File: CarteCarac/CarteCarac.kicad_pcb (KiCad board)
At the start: 4 copper layers, 250 x 130 mm, 30 parts, among them J1 Conn_02x25_Top_Bottom_Mountin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, J2 Conn_02x39_Top_Bottom_Mountin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

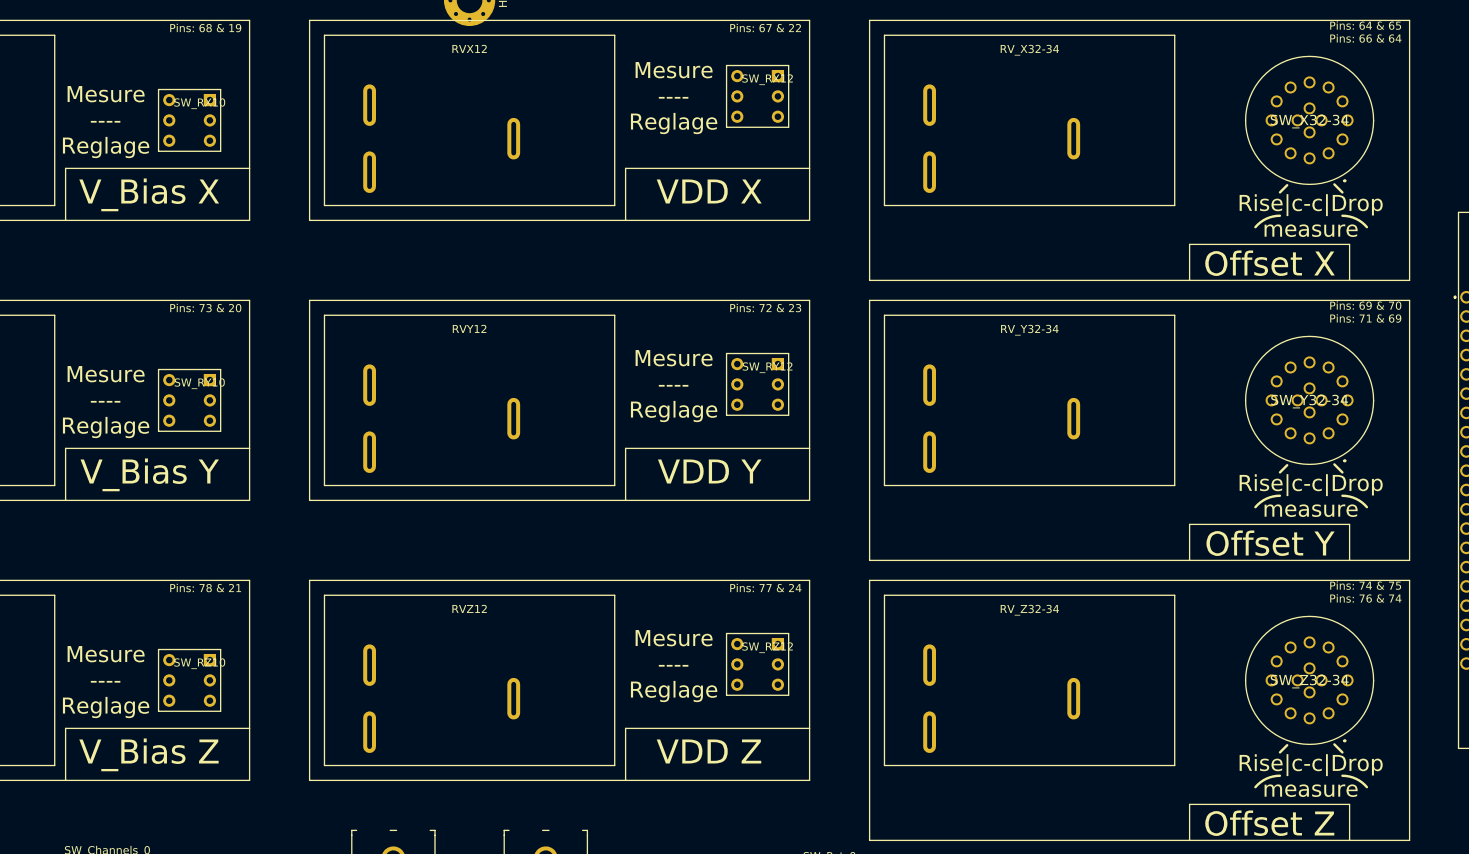
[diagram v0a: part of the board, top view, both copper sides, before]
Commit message: cleaning Pre-routage
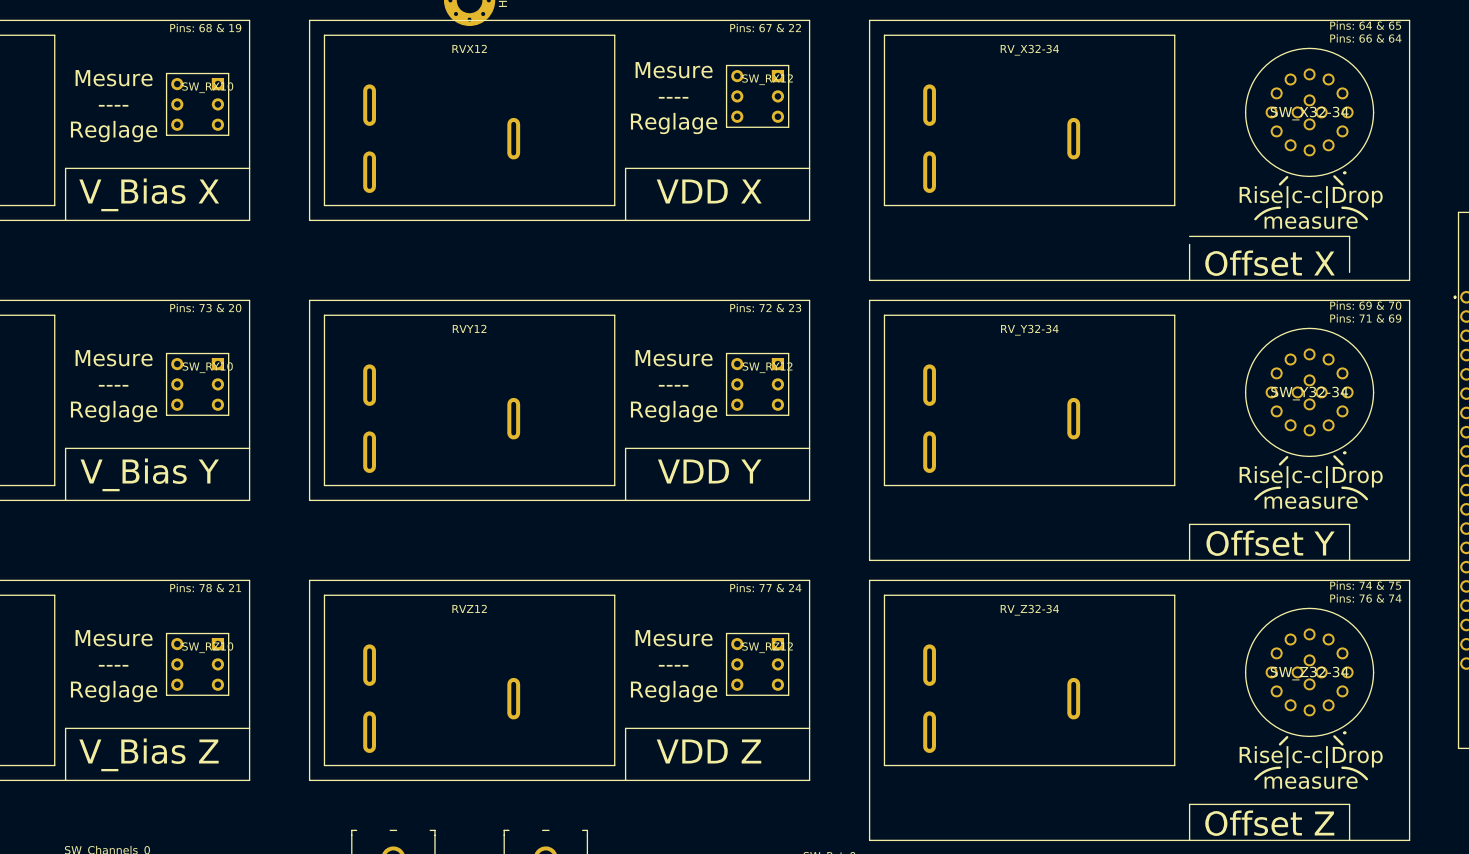
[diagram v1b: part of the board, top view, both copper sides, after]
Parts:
- moved SW_RX10 2.24 mm to (-39.0, -47.0)
- moved SW_RY10 2.24 mm to (-39.0, -12.0)
- moved SW_RZ10 2.24 mm to (-39.0, 23.0)
- moved SW_X32-34 1.00 mm to (100.0, -46.0)
- moved SW_Y32-34 1.00 mm to (100.0, -11.0)
- moved SW_Z32-34 1.00 mm to (100.0, 24.0)
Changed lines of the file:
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@@
   )
   (module LibPersoNadj:Switch_4P3T_MRA403_NKK_Turned30° (layer F.Cu)
-    (at 100 25 180)
+    (at 100 24 180)
     (descr "4P3T MRA403 NKK")
     (tags "Switch 4P3T MRA403 NKK")
@@
   )
   (module LibPersoNadj:Switch_4P3T_MRA403_NKK_Turned30° (layer F.Cu)
-    (at 100 -10 180)
+    (at 100 -11 180)
     (descr "4P3T MRA403 NKK")
     (tags "Switch 4P3T MRA403 NKK")
@@
   )
   (module LibPersoNadj:Switch_4P3T_MRA403_NKK_Turned30° (layer F.Cu)
-    (at 100 -45 180)
+    (at 100 -46 180)
     (descr "4P3T MRA403 NKK")
     (tags "Switch 4P3T MRA403 NKK")
@@
   )
   (module LibPersoNadj:SW_NKK_DPDT_B22AP (layer F.Cu)
-    (at -40 25)
+    (at -39 23)
     (descr "Switch NKK DPDT http://www.nkkswitches.com/pdf/Btoggles.pdf")
     (tags "SWITCH TOGGLE DPDT")
@@
   )
   (module LibPersoNadj:SW_NKK_DPDT_B22AP (layer F.Cu)
-    (at -40 -10)
+    (at -39 -12)
     (descr "Switch NKK DPDT http://www.nkkswitches.com/pdf/Btoggles.pdf")
     (tags "SWITCH TOGGLE DPDT")
@@
   )
   (module LibPersoNadj:SW_NKK_DPDT_B22AP (layer F.Cu)
-    (at -40 -45)
+    (at -39 -47)
     (descr "Switch NKK DPDT http://www.nkkswitches.com/pdf/Btoggles.pdf")
     (tags "SWITCH TOGGLE DPDT")
@@
   (gr_line (start 85 10) (end 85 5.5) (layer F.SilkS) (width 0.12))
   (gr_line (start 85 5.5) (end 105 5.5) (layer F.SilkS) (width 0.12))
-  (gr_line (start 105 -29.5) (end 105 -25) (layer F.SilkS) (width 0.12))
-  (gr_line (start 85 -29.5) (end 105 -29.5) (layer F.SilkS) (width 0.12))
+  (gr_line (start 105 -30.5) (end 105 -26) (layer F.SilkS) (width 0.12))
+  (gr_line (start 85 -30.5) (end 105 -30.5) (layer F.SilkS) (width 0.12))
   (gr_line (start 85 -25) (end 85 -29.5) (layer F.SilkS) (width 0.12))
   (gr_line (start 37.5 -4) (end 14.5 -4) (layer F.SilkS) (width 0.12))
@@
   (gr_line (start -95 -32.5) (end -32.5 -32.5) (layer F.SilkS) (width 0.12))
   (gr_line (start -95 -57.5) (end -95 -32.5) (layer F.SilkS) (width 0.12))
-  (gr_line (start 96.3 -36) (end 97.2 -36.9) (layer F.SilkS) (width 0.3))
-  (gr_text " Rise|c-c|Drop\n measure\n" (at 99.7 -33) (layer F.SilkS)
+  (gr_line (start 96.3 -37) (end 97.2 -37.9) (layer F.SilkS) (width 0.3))
+  (gr_text " Rise|c-c|Drop\n measure\n" (at 99.7 -34) (layer F.SilkS)
     (effects (font (size 2 2) (thickness 0.3)))
   )
-  (gr_line (start 104.1 -36) (end 103.1 -37) (layer F.SilkS) (width 0.3))
-  (gr_arc (start 96.289378 -29.082184) (end 96.289378 -33.082184) (angle -50) (layer F.SilkS) (width 0.3))
-  (gr_arc (start 104.100622 -29.082184) (end 104.100622 -33.082184) (angle 50) (layer F.SilkS) (width 0.3))
-  (gr_line (start 96.3 -1) (end 97.2 -1.9) (layer F.SilkS) (width 0.3))
-  (gr_text " Rise|c-c|Drop\n measure\n" (at 99.7 2) (layer F.SilkS)
+  (gr_line (start 104.1 -37) (end 103.1 -38) (layer F.SilkS) (width 0.3))
+  (gr_arc (start 96.289378 -30.082184) (end 96.289378 -34.082184) (angle -50) (layer F.SilkS) (width 0.3))
+  (gr_arc (start 104.100622 -30.082184) (end 104.100622 -34.082184) (angle 50) (layer F.SilkS) (width 0.3))
+  (gr_line (start 96.3 -2) (end 97.2 -2.9) (layer F.SilkS) (width 0.3))
+  (gr_text " Rise|c-c|Drop\n measure\n" (at 99.7 1) (layer F.SilkS)
     (effects (font (size 2 2) (thickness 0.3)))
   )
-  (gr_line (start 104.1 -1) (end 103.1 -2) (layer F.SilkS) (width 0.3))
-  (gr_arc (start 96.289378 5.917816) (end 96.289378 1.917816) (angle -50) (layer F.SilkS) (width 0.3))
-  (gr_arc (start 104.100622 5.917816) (end 104.100622 1.917816) (angle 50) (layer F.SilkS) (width 0.3))
-  (gr_line (start 96.3 34) (end 97.2 33.1) (layer F.SilkS) (width 0.3))
-  (gr_line (start 104.1 34) (end 103.1 33) (layer F.SilkS) (width 0.3))
-  (gr_arc (start 96.289378 40.917816) (end 96.289378 36.917816) (angle -50) (layer F.SilkS) (width 0.3))
-  (gr_arc (start 104.100622 40.917816) (end 104.100622 36.917816) (angle 50) (layer F.SilkS) (width 0.3))
-  (gr_text " Rise|c-c|Drop\n measure\n" (at 99.7 37) (layer F.SilkS)
+  (gr_line (start 104.1 -2) (end 103.1 -3) (layer F.SilkS) (width 0.3))
+  (gr_arc (start 96.289378 4.917816) (end 96.289378 0.917816) (angle -50) (layer F.SilkS) (width 0.3))
+  (gr_arc (start 104.100622 4.917816) (end 104.100622 0.917816) (angle 50) (layer F.SilkS) (width 0.3))
+  (gr_line (start 96.3 33) (end 97.2 32.1) (layer F.SilkS) (width 0.3))
+  (gr_line (start 104.1 33) (end 103.1 32) (layer F.SilkS) (width 0.3))
+  (gr_arc (start 96.289378 39.917816) (end 96.289378 35.917816) (angle -50) (layer F.SilkS) (width 0.3))
+  (gr_arc (start 104.100622 39.917816) (end 104.100622 35.917816) (angle 50) (layer F.SilkS) (width 0.3))
+  (gr_text " Rise|c-c|Drop\n measure\n" (at 99.7 36) (layer F.SilkS)
     (effects (font (size 2 2) (thickness 0.3)))
   )
@@
     (effects (font (size 2 2) (thickness 0.3)))
   )
-  (gr_text "Mesure\n----\nReglage" (at -50.5 -45) (layer F.SilkS)
+  (gr_text "Mesure\n----\nReglage" (at -49.5 -47) (layer F.SilkS)
     (effects (font (size 2 2) (thickness 0.3)))
   )
-  (gr_text "Mesure\n----\nReglage" (at -50.5 -10) (layer F.SilkS)
+  (gr_text "Mesure\n----\nReglage" (at -49.5 -12) (layer F.SilkS)
     (effects (font (size 2 2) (thickness 0.3)))
   )
@@
     (effects (font (size 3 3) (thickness 0.45)))
   )
-  (gr_text "Mesure\n----\nReglage" (at -50.5 25) (layer F.SilkS)
+  (gr_text "Mesure\n----\nReglage" (at -49.5 23) (layer F.SilkS)
     (effects (font (size 2 2) (thickness 0.3)))
   )
